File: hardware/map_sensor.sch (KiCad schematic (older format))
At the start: 5 parts, among them U4 MPX4250AP1

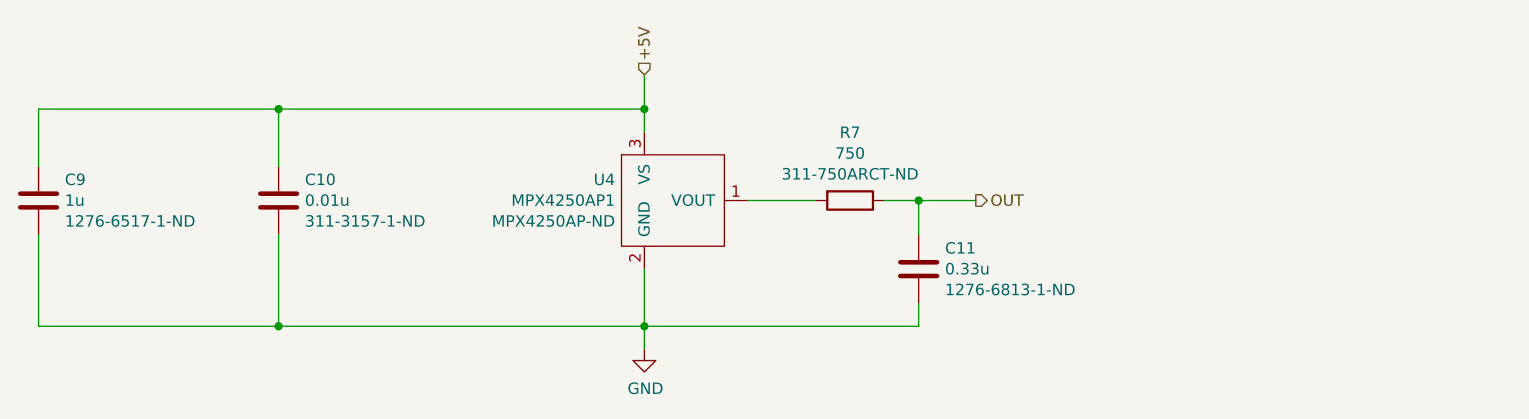
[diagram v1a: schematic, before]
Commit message: hardware rev2 - layout complete
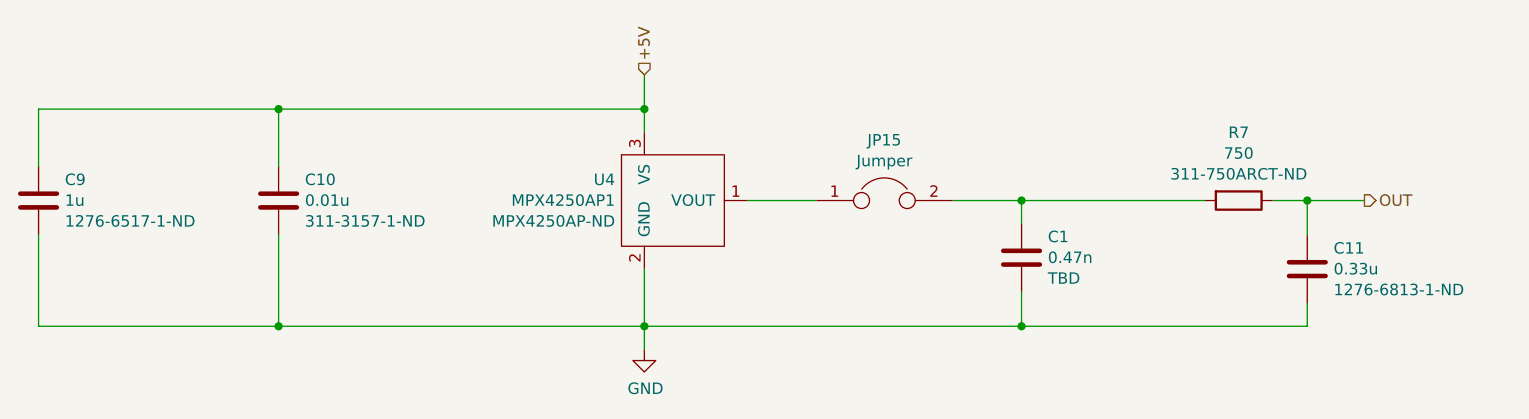
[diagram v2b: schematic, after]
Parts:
- added C1: 0.47n, Capacitors_SMD:C_0805_HandSoldering, symbol Device:C
- added JP15: Jumper, Pin_Headers:Pin_Header_Straight_1x02_Pitch2.54mm, symbol Device:Jumper
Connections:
- net GND: now also C1.2
- net at U4.1 (VOUT): now also JP15.1; no longer R7.2
- new net: C1.1, JP15.2, R7.2
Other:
- moved on the sheet: C11, R7
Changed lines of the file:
@@
 L Device:R R7
 U 1 1 5C653463
-P 6700 3650
-F 0 "R7" V 6403 3650 50  0000 C CNN
-F 1 "750" V 6494 3650 50  0000 C CNN
-F 2 "Resistors_SMD:R_0805_HandSoldering" V 6630 3650 50  0001 C CNN
-F 3 "~" H 6700 3650 50  0001 C CNN
-F 4 "311-750ARCT-ND" V 6585 3650 50  0000 C CNN "DIGIKEY"
-	1    6700 3650
+P 8400 3650
+F 0 "R7" V 8103 3650 50  0000 C CNN
+F 1 "750" V 8194 3650 50  0000 C CNN
+F 2 "Resistors_SMD:R_0805_HandSoldering" V 8330 3650 50  0001 C CNN
+F 3 "~" H 8400 3650 50  0001 C CNN
+F 4 "311-750ARCT-ND" V 8285 3650 50  0000 C CNN "DIGIKEY"
+	1    8400 3650
 	0    1    1    0
 $EndComp
-Wire Wire Line
-	6250 3650 6550 3650
 $Comp
 L Device:C C11
 U 1 1 5C6534D1
-P 7000 3950
-F 0 "C11" H 7115 4041 50  0000 L CNN
-F 1 "0.33u" H 7115 3950 50  0000 L CNN
-F 2 "Capacitors_SMD:C_0805_HandSoldering" H 7038 3800 50  0001 C CNN
-F 3 "~" H 7000 3950 50  0001 C CNN
-F 4 "1276-6813-1-ND" H 7115 3859 50  0000 L CNN "DIGIKEY"
-	1    7000 3950
+P 8700 3950
+F 0 "C11" H 8815 4041 50  0000 L CNN
+F 1 "0.33u" H 8815 3950 50  0000 L CNN
+F 2 "Capacitors_SMD:C_0805_HandSoldering" H 8738 3800 50  0001 C CNN
+F 3 "~" H 8700 3950 50  0001 C CNN
+F 4 "1276-6813-1-ND" H 8815 3859 50  0000 L CNN "DIGIKEY"
+	1    8700 3950
 	1    0    0    -1
 $EndComp
 Wire Wire Line
-	6850 3650 7000 3650
+	8550 3650 8700 3650
 Wire Wire Line
-	7000 3650 7000 3800
-Text HLabel 7250 3650 2    50   Output ~ 0
+	8700 3650 8700 3800
+Text HLabel 8950 3650 2    50   Output ~ 0
 OUT
 Wire Wire Line
-	7000 3650 7250 3650
-Connection ~ 7000 3650
+	8700 3650 8950 3650
+Connection ~ 8700 3650
 Wire Wire Line
 	5800 3100 5800 3250
@@
 Connection ~ 4200 4200
 Wire Wire Line
-	7000 4100 7000 4200
+	8700 4100 8700 4200
 Wire Wire Line
-	7000 4200 5800 4200
+	8700 4200 7450 4200
 Text HLabel 5800 3100 1    50   Input ~ 0
 +5V
+$Comp
+L Device:C C1
+U 1 1 5CFE504F
+P 7450 3900
+F 0 "C1" H 7565 3991 50  0000 L CNN
+F 1 "0.47n" H 7565 3900 50  0000 L CNN
+F 2 "Capacitors_SMD:C_0805_HandSoldering" H 7488 3750 50  0001 C CNN
+F 3 "~" H 7450 3900 50  0001 C CNN
+F 4 "TBD" H 7565 3809 50  0000 L CNN "DIGIKEY"
+	1    7450 3900
+	1    0    0    -1
+$EndComp
+Wire Wire Line
+	7450 3750 7450 3650
+Wire Wire Line
+	7450 3650 8250 3650
+Wire Wire Line
+	7450 4050 7450 4200
+Connection ~ 7450 4200
+Wire Wire Line
+	7450 4200 5800 4200
+$Comp
+L Device:Jumper JP?
+U 1 1 5D01020C
+P 6850 3650
+AR Path="/5D01020C" Ref="JP?"  Part="1"
+AR Path="/5C653342/5D01020C" Ref="JP15"  Part="1"
+F 0 "JP15" H 6850 3914 50  0000 C CNN
+F 1 "Jumper" H 6850 3823 50  0000 C CNN
+F 2 "Pin_Headers:Pin_Header_Straight_1x02_Pitch2.54mm" H 6850 3650 50  0001 C CNN
+F 3 "~" H 6850 3650 50  0001 C CNN
+	1    6850 3650
+	1    0    0    -1
+$EndComp
+Wire Wire Line
+	6250 3650 6550 3650
+Wire Wire Line
+	7150 3650 7450 3650
+Connection ~ 7450 3650
 $EndSCHEMATC
